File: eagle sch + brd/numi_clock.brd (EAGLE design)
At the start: 100 x 80 mm, 40 parts, among them IC1 MAX7219CWG, IC2 MEGA8-AI, IC4 DS1307Z, Q1 12 MHz, Q2 32kHz, X2 MINI-USB-UX60-MB-5S8

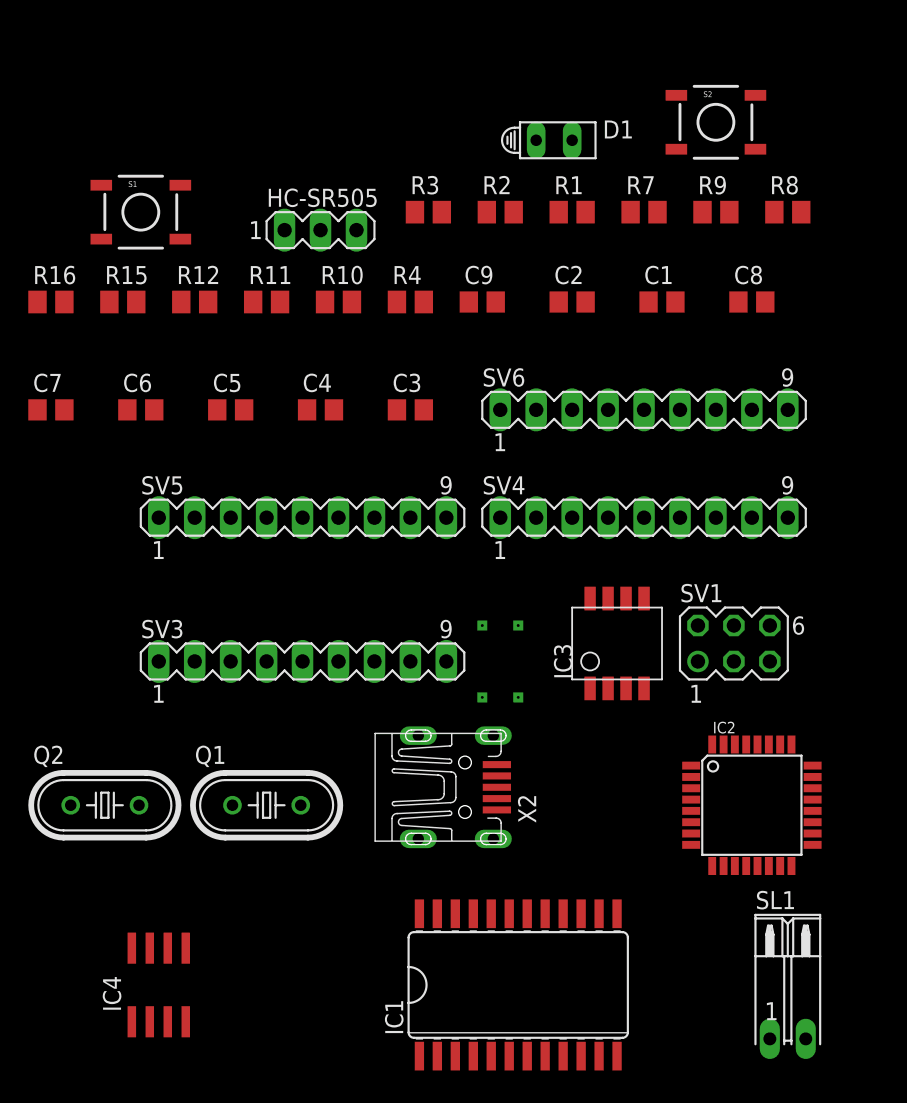
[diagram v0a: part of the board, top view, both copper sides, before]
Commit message: Fixes #1
Fixes #1
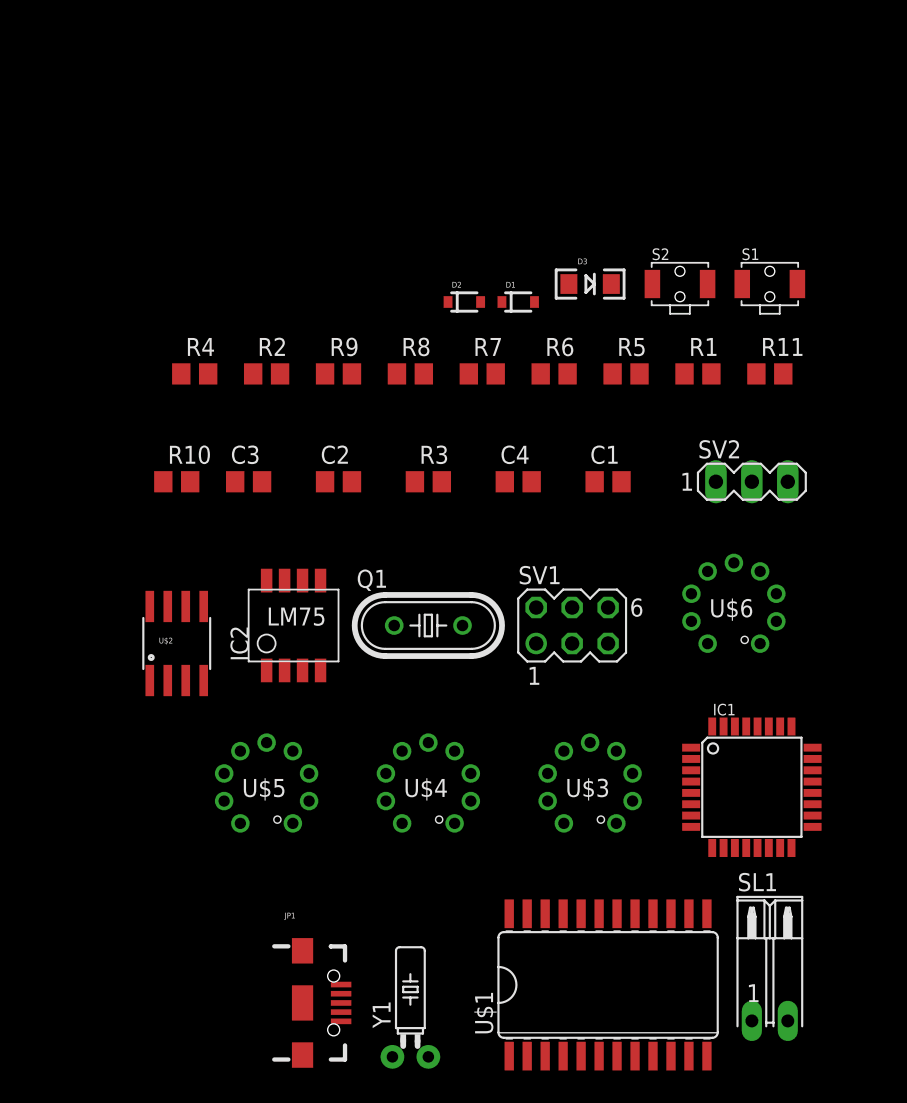
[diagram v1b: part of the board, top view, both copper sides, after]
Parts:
- removed C5, C6, C7, C8: 100nF, resistor:C0805
- removed C9: 27pF, resistor:C0805
- removed HC-SR505: (no value), con-lstb:MA03-1
- removed IC3: (no value), lm75:SO8_LM75
- removed IC4: DS1307Z, ds1307_pcf8583:SOIC8
- removed Q2: 32kHz, crystal:HC49U-V
- removed R12: 26k, resistor:M0805
- removed R15, R16: 10K, resistor:M0805
- removed SV3, SV4, SV5, SV6: (no value), con-lstb:MA09-1
- removed X2: MINI-USB-UX60-MB-5S8, con-hirose:UX60-MB-5S8
- added D2: 3.6V, SparkFun-DiscreteSemi:SOD-323
- added D3: red, SparkFun-LED:LED-1206
- added JP1: micro-usb, SparkFun-Connectors:USB-B-MICRO-SMD_V03
- added SV2: HC-SR505, con-lstb:MA03-1
- added U$1: MAX7219CWG, max7219:SO24L
- added U$2: DS1307SO8, SparkFun-FreqCtrl:SO08
- added U$3, U$4, U$5, U$6: IV-9, domestichacks:IV-9
- added Y1: 32.768kHz, SparkFun-FreqCtrl:TC26H
- C1: value 27pF -> 100nF; device resistor:C0805 -> rcl:C0805
- C2, C4: device resistor:C0805 -> rcl:C0805
- C3: value 100nF -> 27pF; device resistor:C0805 -> rcl:C0805
- D1: value RED -> 3.6V; device display-hp:HLMP6 -> SparkFun-DiscreteSemi:SOD-323
- IC1: value MAX7219CWG -> MEGA8-AI; device max7219:SO24L -> atmel:TQFP32-08
- IC2: value MEGA8-AI -> LM75; device atmel:TQFP32-08 -> lm75:SO8_LM75
- Q1: value 12 MHz -> 12MHz; device crystal:HC49U-V -> crystal:HC49/S
- R1, R2: device resistor:M0805 -> rcl:R0805
- R10, R8, R9: value 10K -> 10k; device resistor:M0805 -> rcl:R0805
- R11: value 10K -> 23k; device resistor:M0805 -> rcl:R0805
- R3: value 68 -> 1.8k; device resistor:M0805 -> rcl:R0805
- R4: value 1.8K -> 68; device resistor:M0805 -> rcl:R0805
- R5, R6: value 3v6 -> 10k; device e-halbleiter:Z-DIODE -> rcl:R0805
- R7: value 330 -> 10k; device resistor:M0805 -> rcl:R0805
- S1, S2: value SWITCH-MOMENTARY-2SMD -> SWITCH-MOMENTARY-2TACTILE-SWITCH-SMD-RIGHT-ANGLE; device SparkFun-Electromechanical:TACTILE-SWITCH-SMD -> SparkFun-Electromechanical:TACTILE_SWITCH-SMD-RIGHT-ANGLE
- SL1: value (none) -> VBATT
- SV1: value (none) -> SPI
- moved S1 44.7 mm to (-16.5, 55.9)
- moved R11 35.9 mm to (-16.5, 49.5)
- moved IC2 35.4 mm to (-50.8, 31.8)
- moved R9 29.0 mm to (-47.0, 49.5)
- moved R8 29.0 mm to (-41.9, 49.5)
- moved R5 21.7 mm to (-26.7, 49.5)
- moved IC1 21.6 mm to (-17.8, 20.3)
- moved R6 20.9 mm to (-31.8, 49.5)
- moved C2 20.8 mm to (-47.0, 41.9)
- moved R2 20.1 mm to (-52.1, 49.5)
- moved R3 19.1 mm to (-40.6, 41.9)
- moved Q1 17.1 mm to (-40.6, 31.8)
- moved R10 17.1 mm to (-58.4, 41.9)
- moved R7 16.2 mm to (-36.8, 49.5)
- moved R4 16.1 mm to (-57.1, 49.5)
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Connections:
- removed net CLK: IC1.13
- removed net N$12: R1.1
- removed net N$14: C9.1, IC3.8
- removed net N$15: IC2.4
- removed net N$16: R11.2
- removed net N$17: IC1.18, R12.2
- removed net N$18: IC2.8
- removed net N$19: IC2.7
- removed net N$20: IC2.1
- removed net N$21: R9.2
- removed net N$22: R8.1
- removed net N$23: R6.A
- removed net N$24: R5.C
- removed net N$26: R6.C
- removed net N$28: SL1.2
- removed net N$29: C2.1
- removed net N$30: D1.K, R7.1
- removed net N$31: SV1.2
- removed net N$32: R1.2
- removed net N$35: IC4.2, Q2.1
- removed net N$36: IC4.1, Q2.2
- removed net N$39: IC3.4
- removed net N$42: IC1.4, IC1.9
- removed net N$45: SV3.6
- removed net N$48: IC3.5
- removed net N$6: R2.1, X2.3
- new net N$10: IC1.1, R2.2
- new net N$8: D1.C, JP1.D-1, R2.1, R3.2
- net +3V3: now also R5.1, R6.1, R7.1, R9.1, S1.1, SL1.2, U$2.3; no longer IC4.3, R11.1, S2.1
- net +5V: now also D3.A, IC1.18, IC1.20, IC1.4, IC1.6, IC2.8, JP1.VBUS1, R1.2, R10.1, R11.1, R3.1, R8.1, SV1.2, SV2.1, U$1.19, U$2.8; no longer C3.2, C5.2, C6.2, C8.2, D1.A, IC1.19, IC2.18, IC2.20, IC2.6, IC4.8, R12.1, R15.1, R16.1, R4.1, X2.1
- net A: now also U$1.14, U$3.5, U$4.5, U$5.5, U$6.5; no longer IC1.14, SV3.8, SV4.8, SV5.8, SV6.8
- net B: now also U$1.16, U$3.3, U$4.3, U$5.3, U$6.3; no longer IC1.16, SV3.7, SV4.7, SV5.7, SV6.7
- net C: now also U$1.20, U$3.4, U$4.4, U$5.4, U$6.4; no longer IC1.20, SV4.6, SV5.6, SV6.6
- net CS: now also IC1.24, U$1.12; no longer IC1.12, IC2.24
- net D: now also U$1.23, U$3.8, U$4.8, U$5.8, U$6.8; no longer IC1.23, SV3.5, SV4.5, SV5.5, SV6.5
- net DIG0: now also R9.2, U$1.2, U$6.1; no longer IC1.2, SV3.9
- net DIG1: now also R7.2, U$1.11, U$5.1; no longer IC1.11
- net DIG2: now also R6.2, U$1.6, U$4.1; no longer IC1.6, SV5.9
- net DIG3: now also R5.2, U$1.7, U$3.1; no longer IC1.7, R8.2, SV6.9
- net DP: now also U$1.22, U$3.2, U$4.2, U$5.2, U$6.2; no longer IC1.22, SV3.1, SV4.1, SV5.1, SV6.1
- net E: now also U$1.21, U$3.9, U$4.9, U$5.9, U$6.9; no longer IC1.21, SV3.4, SV4.4, SV5.4, SV6.4
- net F: now also U$1.15, U$3.6, U$4.6, U$5.6, U$6.6; no longer IC1.15, SV3.3, SV4.3, SV5.3, SV6.3
- net G: now also U$1.17, U$3.7, U$4.7, U$5.7, U$6.7; no longer IC1.17, SV3.2, SV4.2, SV5.2, SV6.2
- net GND: now also C2.1, D1.A, D2.A, D3.C, IC1.21, IC1.3, IC1.5, IC2.4, IC2.6, IC2.7, JP1.GND1, JP1.ID1, S1.2, S2.2, SV2.3, U$1.4, U$1.9, U$2.4; no longer C5.1, C6.1, C7.1, C8.1, C9.2, HC-SR505.3, IC2.21, IC2.3, IC3.6, IC3.7, IC4.4, R5.A, R7.2, S1.3, S2.3
- net HC: now also IC1.23, SV2.2; no longer HC-SR505.2, IC2.23
- net MISO: now also IC1.16
- net MOSI: now also IC1.15, U$1.1; no longer IC1.1
- net N$1: now also C2.2, IC1.7; no longer C1.2
- net N$2: now also C3.2, IC1.8; no longer C2.2
- net N$3: now also R11.2, U$1.18; no longer HC-SR505.1
- net N$4: now also U$2.1, Y1.2; no longer R3.2
- net N$5: now also U$2.2, Y1.1; no longer S1.1
- net N$7: now also D2.C, JP1.D+1, R4.1; no longer R3.1, R4.2, X2.2
- net N$9: now also IC1.32, R4.2; no longer IC2.32, R2.2
- net RESET: now also C1.2, IC1.29, R1.1, S2.1; no longer C7.2, IC2.29
- net SCK: now also IC1.17, U$1.13
- net SCL: now also IC2.2, R10.2, U$2.6; no longer IC2.28, IC3.2, IC4.6, R16.2
- net SDA: now also IC2.1, R8.2, U$2.5; no longer IC2.27, IC3.1, IC4.5, R15.2
